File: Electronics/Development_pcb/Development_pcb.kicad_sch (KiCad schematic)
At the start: 11 parts, among them J1 TF-Luna, J2 Pan, J3 Tilt, J4 MP3, Q1 NPN, U1 ESP32-S3-DEVKIT:C-1-N16R8, U2 MP3-TF-16P

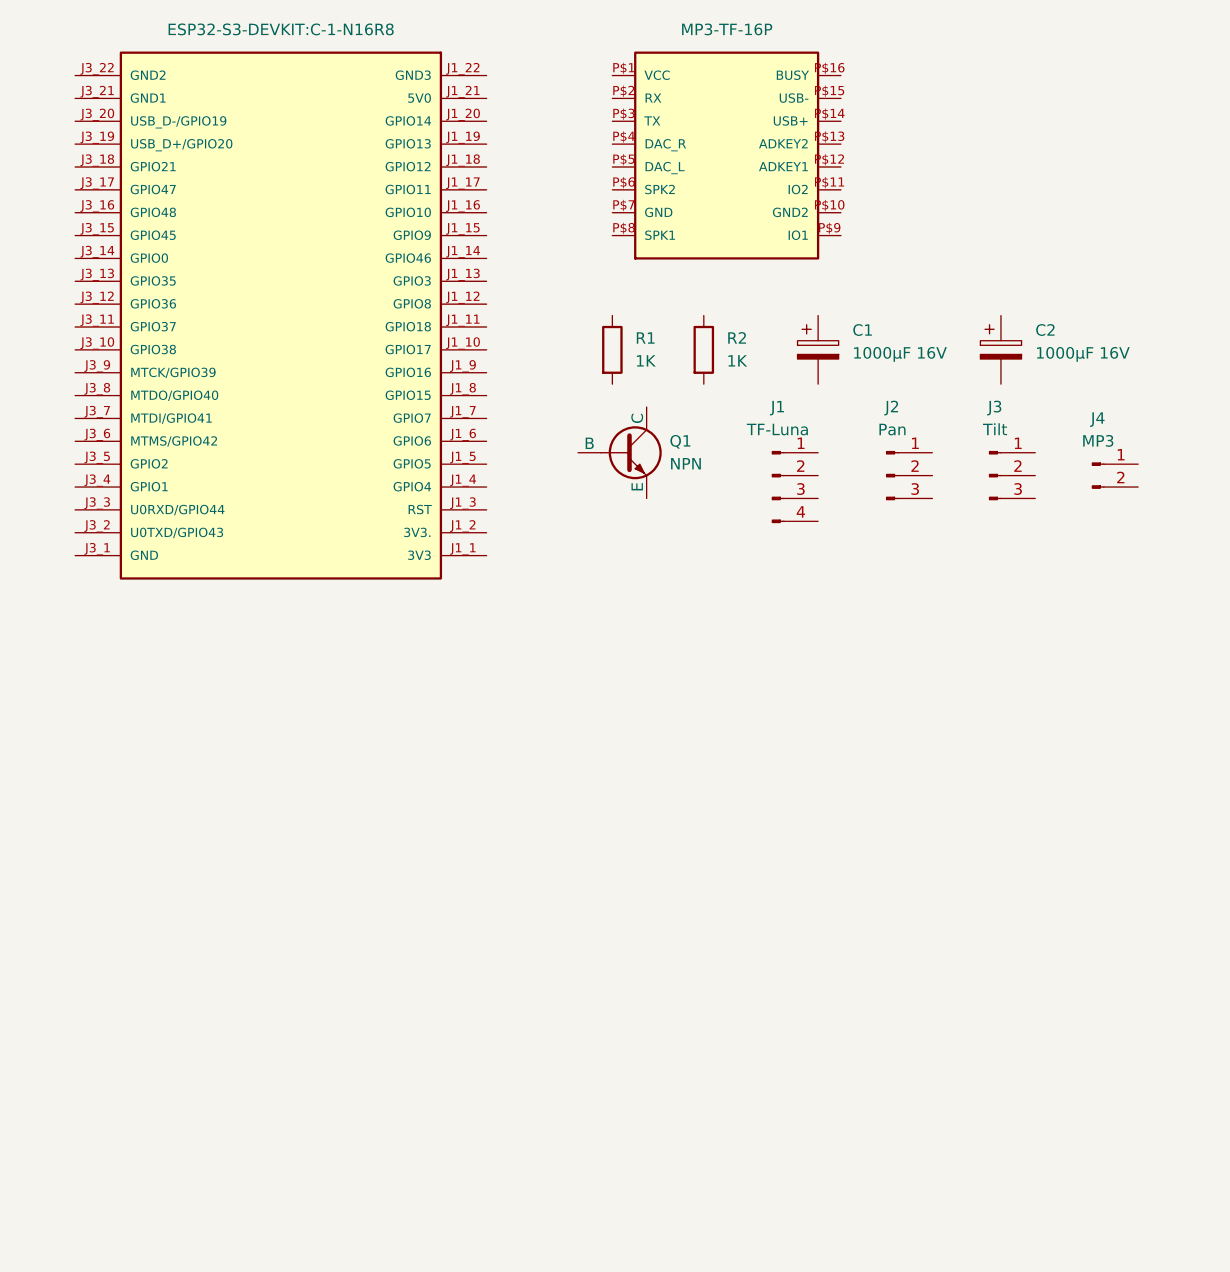
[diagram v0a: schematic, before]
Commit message: Refactor code structure for improved readability and maintainability
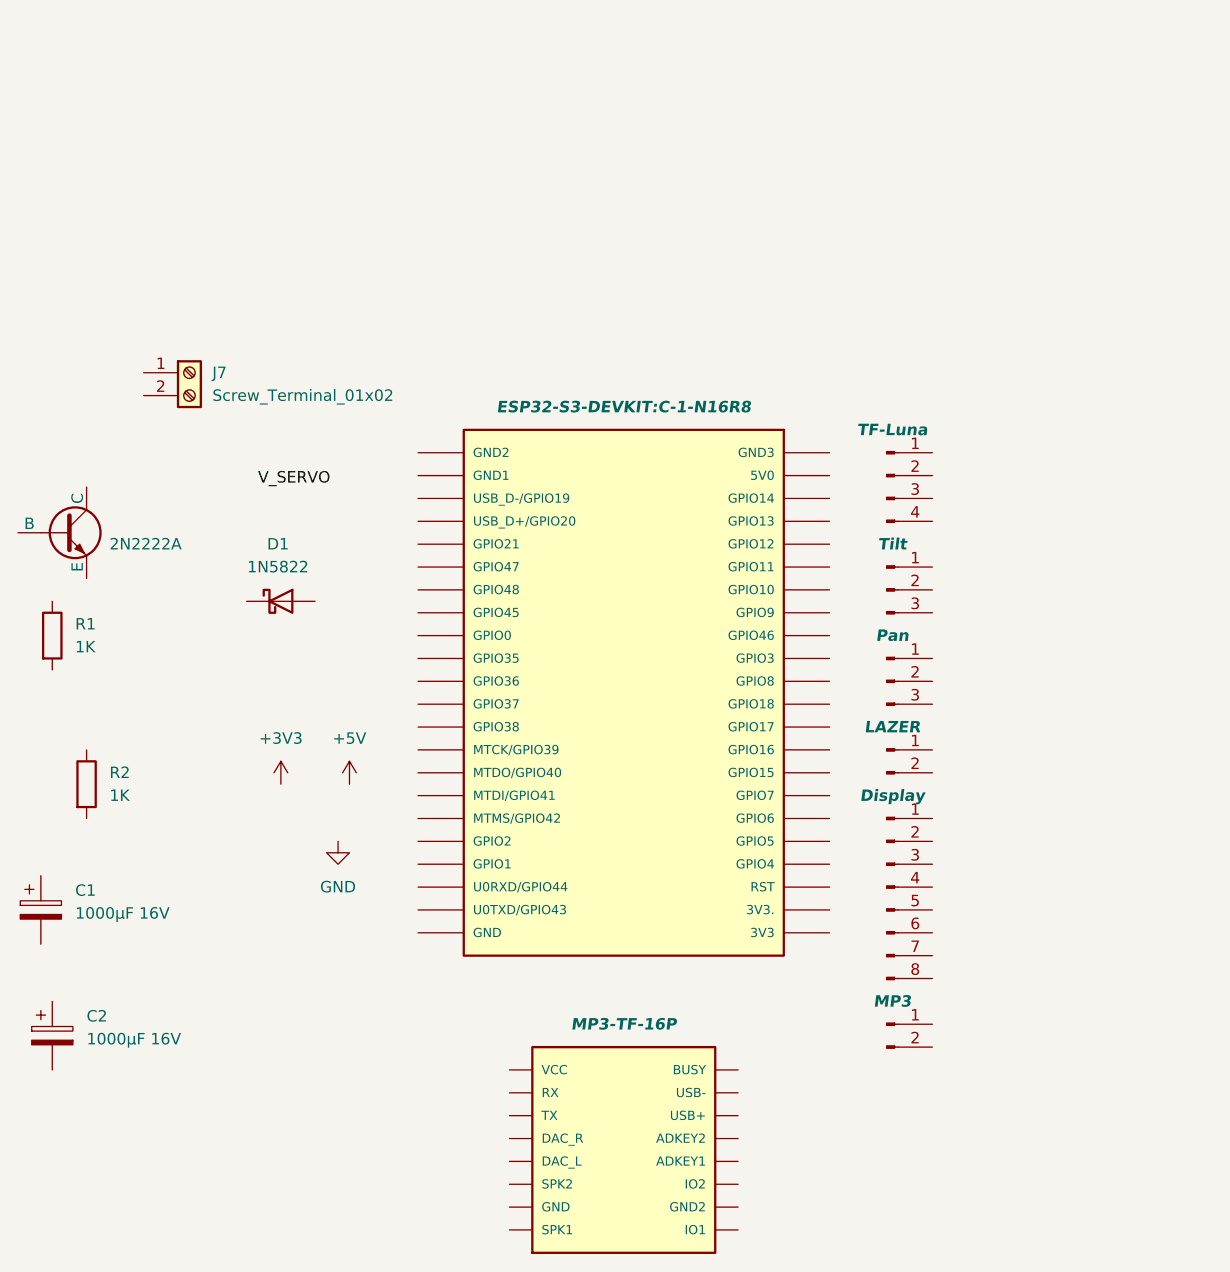
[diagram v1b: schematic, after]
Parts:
- added D1: 1N5822, Diode_THT:D_DO-201AD_P15.24mm_Horizontal, symbol Diode:1N5822
- added J5: Display, symbol Connector:Conn_01x08_Pin
- added J6: LAZER, symbol Connector:Conn_01x02_Pin
- added J7: Screw_Terminal_01x02, symbol Connector:Screw_Terminal_01x02
- Q1: value NPN -> 2N2222A
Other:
- moved on the sheet: C1, C2, R1, R2

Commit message: Refactor code structure for improved readability and maintainability
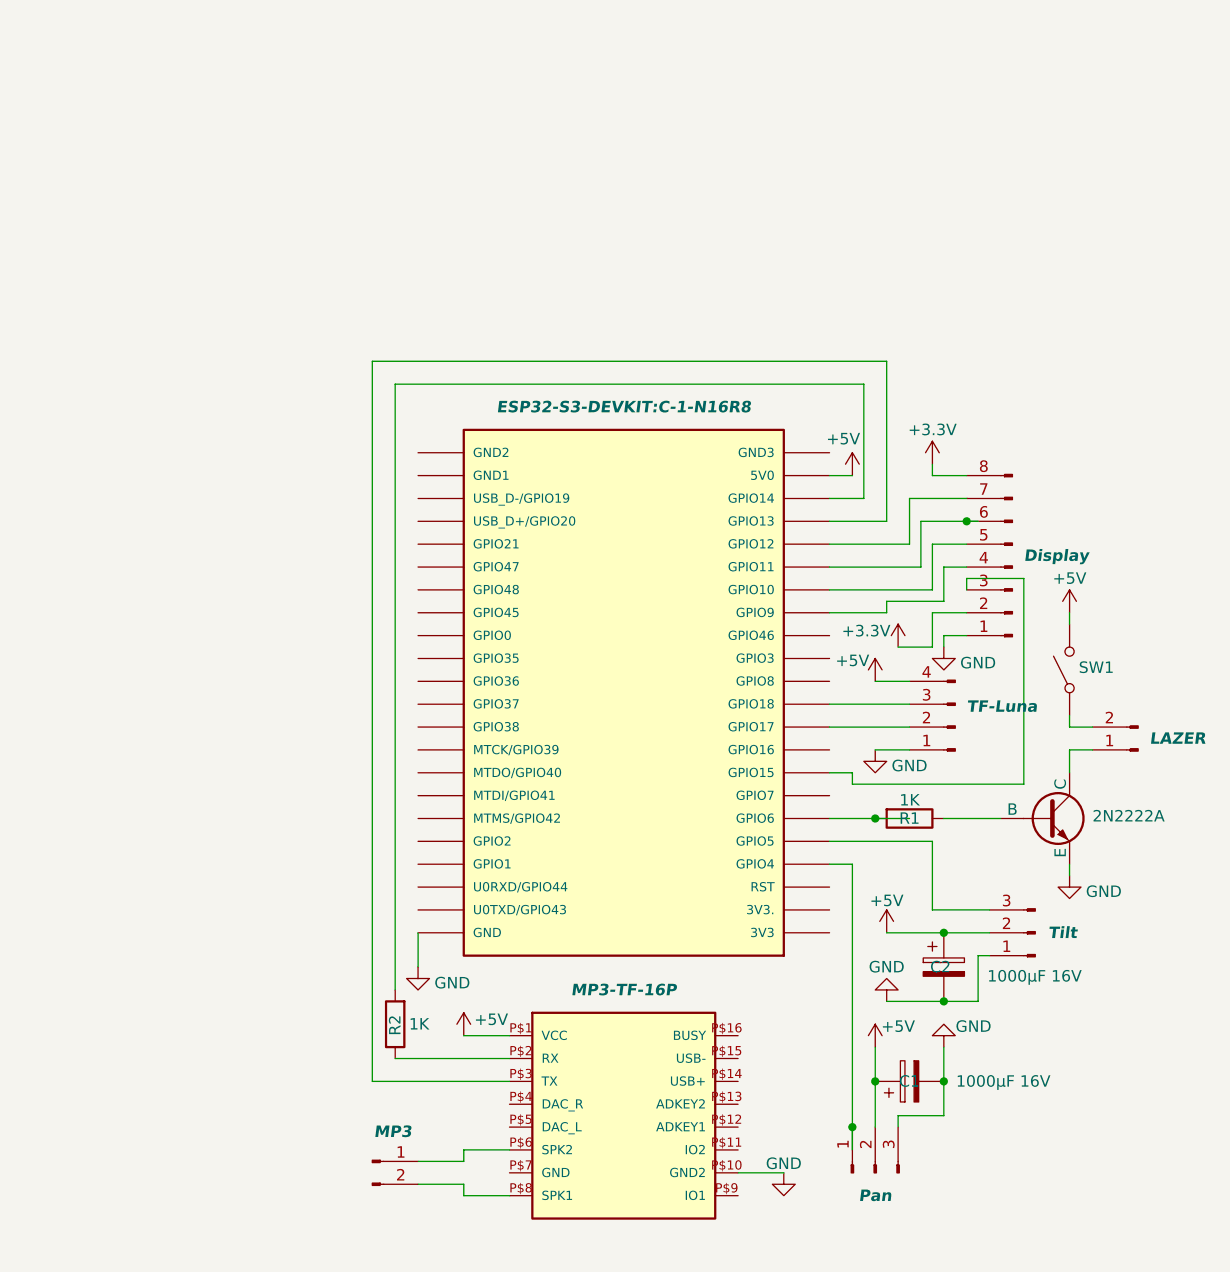
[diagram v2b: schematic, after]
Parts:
- removed D1: 1N5822, Diode_THT:D_DO-201AD_P15.24mm_Horizontal, symbol Diode:1N5822
- removed J7: Screw_Terminal_01x02, symbol Connector:Screw_Terminal_01x02
- added SW1: SW_SPST, Connector_PinHeader_2.54mm:PinHeader_1x02_P2.54mm_Vertical, symbol Switch:SW_SPST
- C1, C2: footprint (none) -> Capacitor_THT:CP_Radial_D10.0mm_P5.00mm
- J1: footprint (none) -> Connector_PinHeader_2.54mm:PinHeader_1x04_P2.54mm_Vertical
- J2, J3: footprint (none) -> Connector_PinHeader_2.54mm:PinHeader_1x03_P2.54mm_Vertical
- J4, J6: footprint (none) -> Connector_PinHeader_2.54mm:PinHeader_1x02_P2.54mm_Vertical
- J5: footprint (none) -> Connector_PinHeader_2.54mm:PinHeader_1x08_P2.54mm_Vertical
- Q1: footprint (none) -> Package_TO_SOT_THT:TO-92_Inline
- R1, R2: footprint (none) -> Resistor_THT:R_Axial_DIN0207_L6.3mm_D2.5mm_P7.62mm_Horizontal
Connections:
- net +5V: now also C1.1, C2.1, J1.4 (Pin_4), J2.2 (Pin_2), J3.2 (Pin_2), U1.J1_21 (5V0), U2.P$1 (VCC), SW1.2 (B)
- net GND: now also C1.2, C2.2, J1.1 (Pin_1), J2.3 (Pin_3), J3.1 (Pin_1), J5.1 (Pin_1), Q1.3 (E), U1.J3_1 (GND), U2.P$10 (GND2)
- net at Q1.1 (C): now also J6.1 (Pin_1)
- net at Q1.2 (B): now also R1.1
- net at R1.2: now also U1.J1_6 (GPIO6)
- net +3.3V: now reaches J5.2 (Pin_2)
- net +3.3V: now also J5.8 (Pin_8)
- net at J5.3 (Pin_3): now also U1.J1_8 (GPIO15)
- net at J5.4 (Pin_4): now also U1.J1_15 (GPIO9)
- net at J5.5 (Pin_5): now also U1.J1_16 (GPIO10)
- net at J5.6 (Pin_6): now also U1.J1_17 (GPIO11)
- net at J5.7 (Pin_7): now also U1.J1_18 (GPIO12)
- net at J2.1 (Pin_1): now also U1.J1_4 (GPIO4)
- net at J4.1 (Pin_1): now also U2.P$6 (SPK2)
- net at J4.2 (Pin_2): now also U2.P$8 (SPK1)
- net at U2.P$2 (RX): now also R2.1
- net at U2.P$3 (TX): now also U1.J1_19 (GPIO13)
- net at J6.2 (Pin_2): now also SW1.1 (A)
- net at U1.J1_10 (GPIO17): now also J1.2 (Pin_2)
- net at U1.J1_11 (GPIO18): now also J1.3 (Pin_3)
- net at U1.J1_20 (GPIO14): now also R2.2
- net at U1.J1_5 (GPIO5): now also J3.3 (Pin_3)
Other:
- company: (none) -> Artyom Kiselhof
- title: (none) -> MISA_PCB
- moved on the sheet: C1, C2, R1, R2
